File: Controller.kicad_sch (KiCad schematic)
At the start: 28 parts, among them IC3 STM32H563VGT6, U4 BMI088

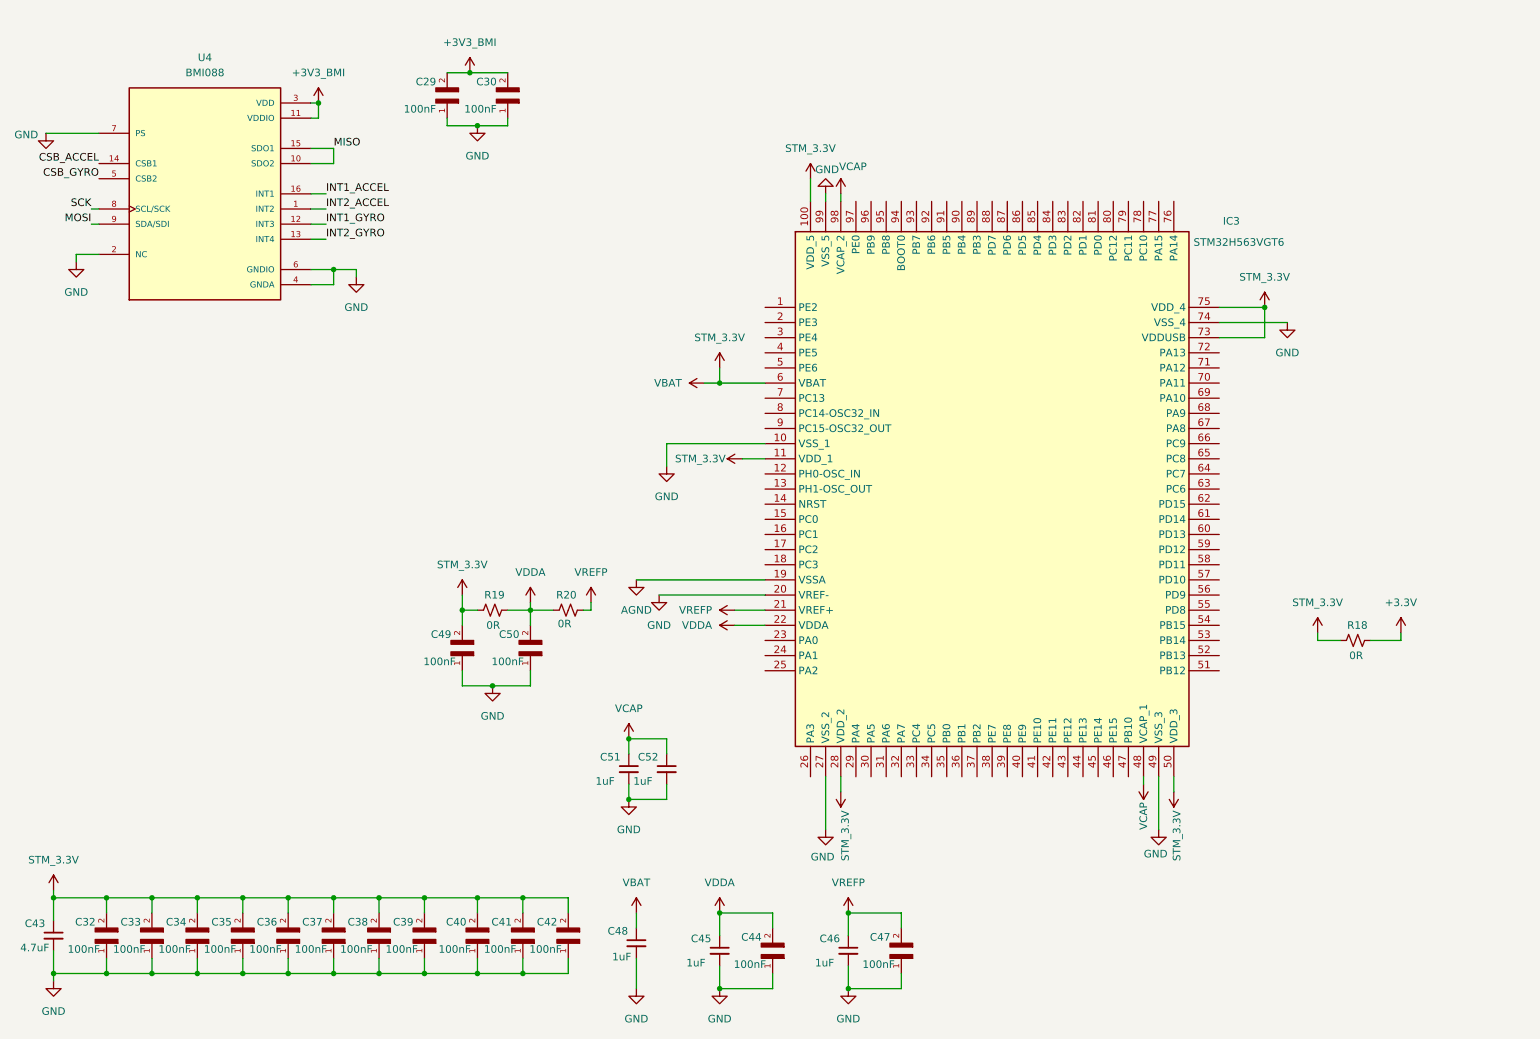
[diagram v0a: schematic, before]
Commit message: new update
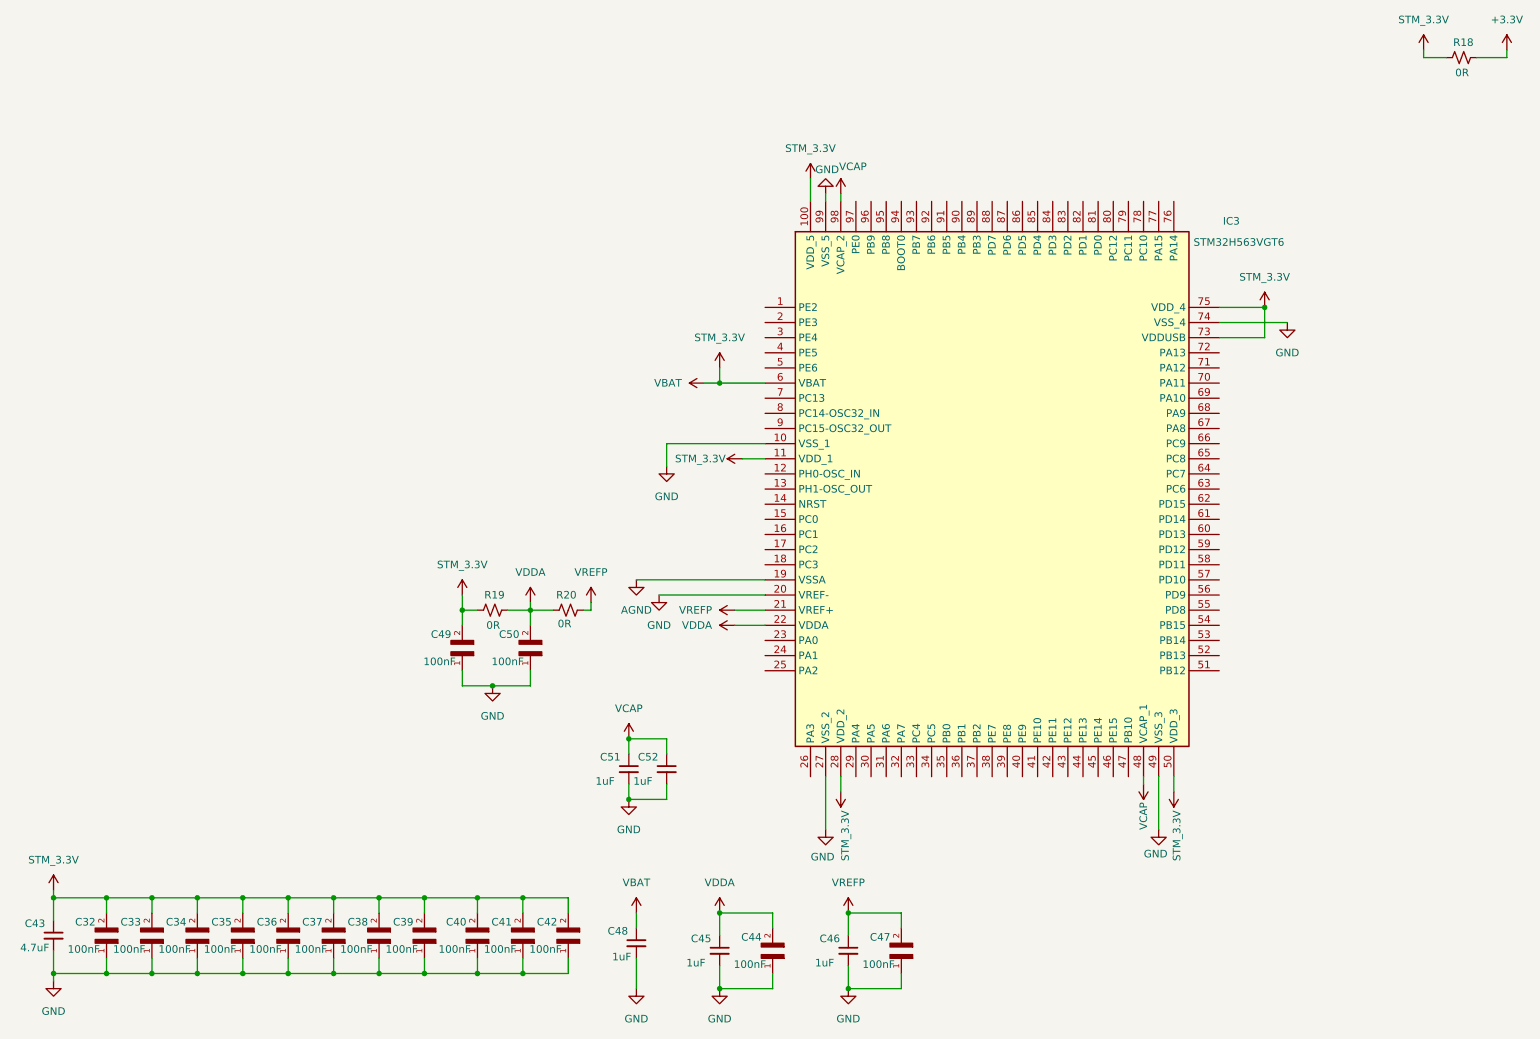
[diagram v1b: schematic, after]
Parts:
- removed C29, C30: 100nF, C0402C104K4RAC:CAPC1005X55N, symbol C0402C104K4RAC:C0402C104K4RAC
- removed U4: BMI088, Module:PQFN50P450X300X100-16N, symbol BMI088:BMI088
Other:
- moved on the sheet: R18

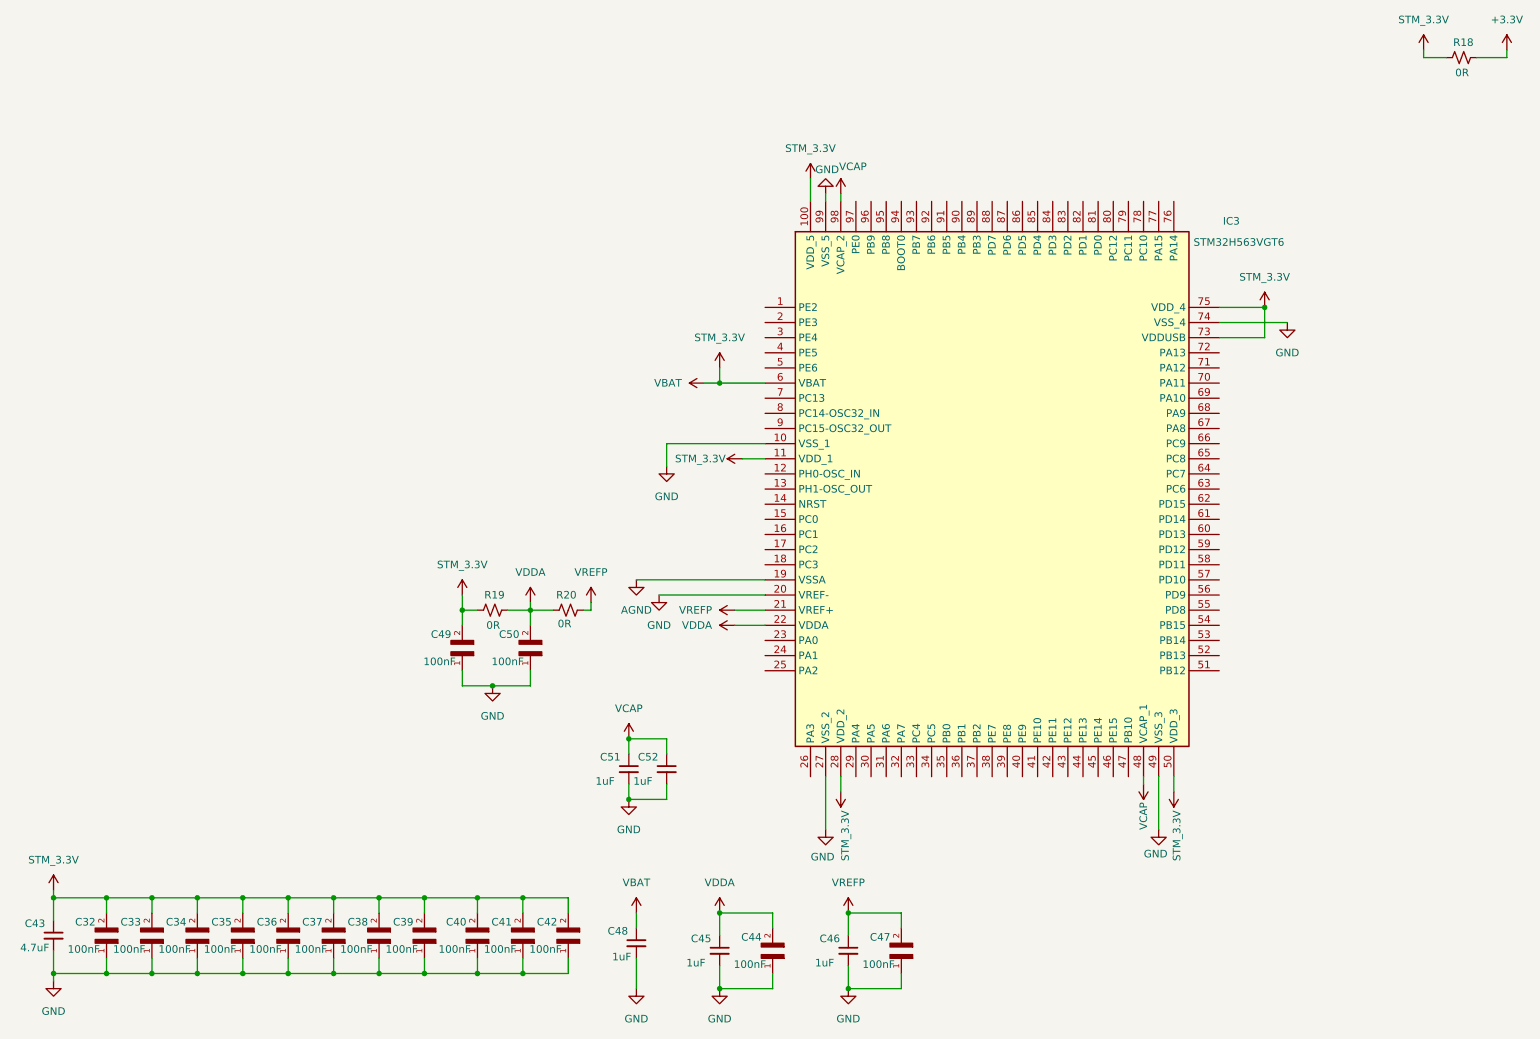
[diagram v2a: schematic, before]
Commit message: new
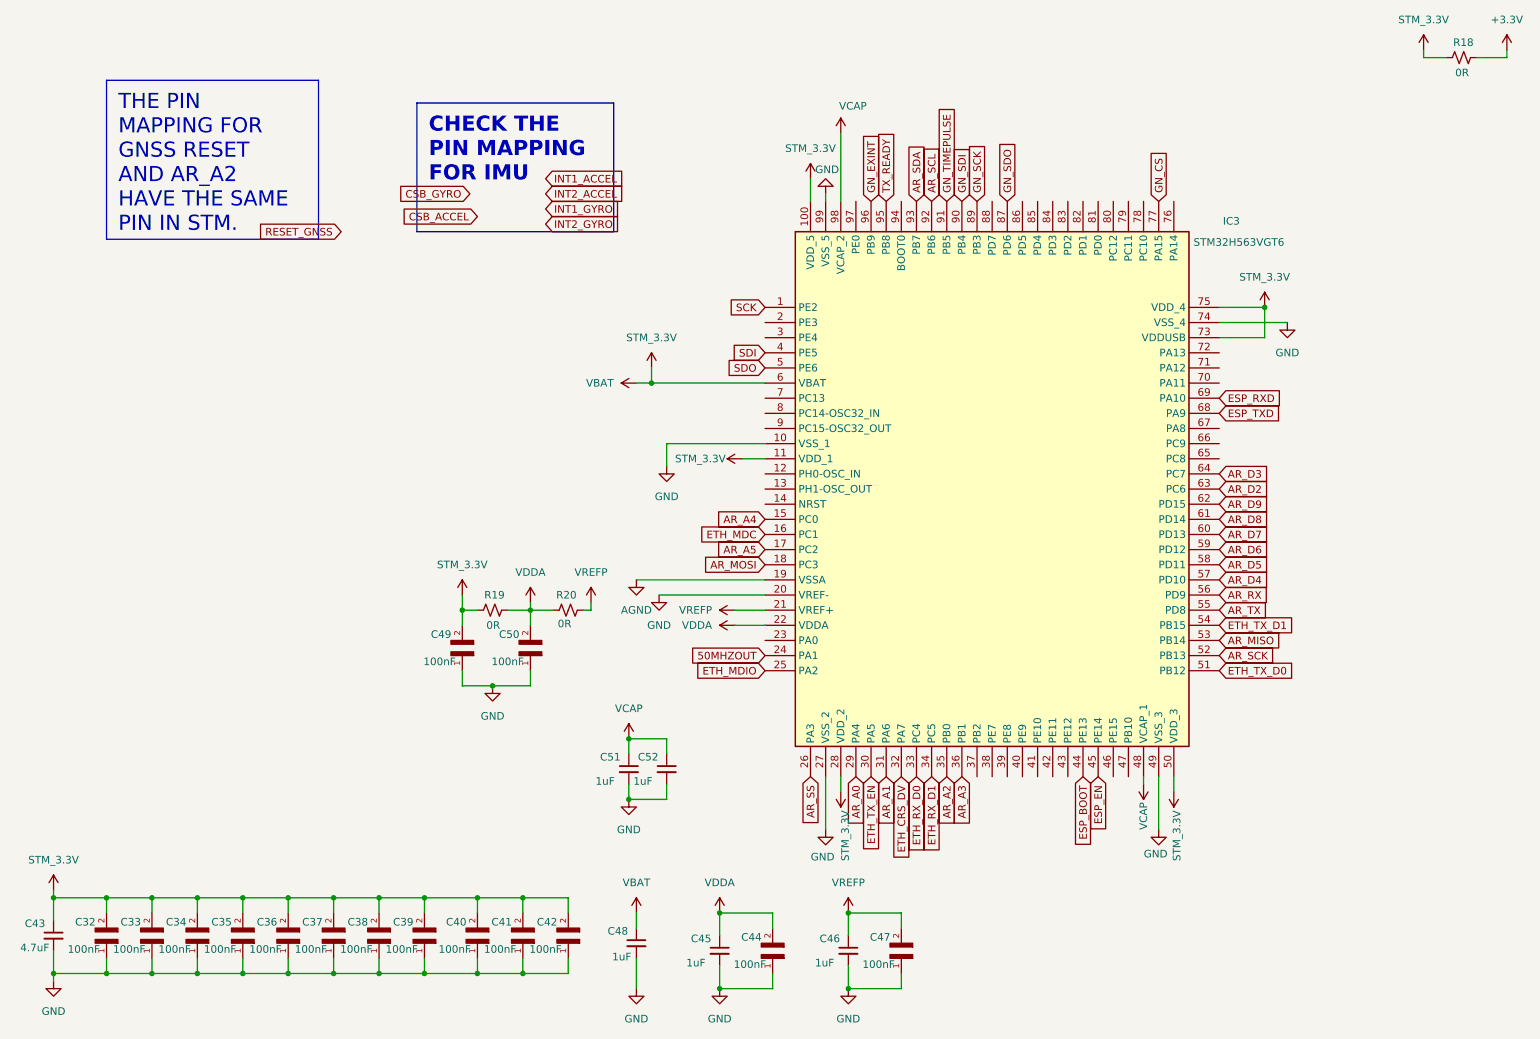
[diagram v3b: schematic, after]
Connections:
- net SCK: now reaches IC3.1 (PE2)
- net AR_A4: now reaches IC3.15 (PC0)
- net ETH_MDC: now reaches IC3.16 (PC1)
- net AR_A5: now reaches IC3.17 (PC2)
- net AR_MOSI: now reaches IC3.18 (PC3)
- net 50MHZOUT: now reaches IC3.24 (PA1)
- net ETH_MDIO: now reaches IC3.25 (PA2)
- net AR_SS: now reaches IC3.26 (PA3)
- net AR_A0: now reaches IC3.29 (PA4)
- net ETH_TX_EN: now reaches IC3.30 (PA5)
- net AR_A1: now reaches IC3.31 (PA6)
- net ETH_CRS_DV: now reaches IC3.32 (PA7)
- net ETH_RX_D0: now reaches IC3.33 (PC4)
- net ETH_RX_D1: now reaches IC3.34 (PC5)
- net AR_A2: now reaches IC3.35 (PB0)
- net AR_A3: now reaches IC3.36 (PB1)
- net SDI: now reaches IC3.4 (PE5)
- net ESP_BOOT: now reaches IC3.44 (PE13)
- net ESP_EN: now reaches IC3.45 (PE14)
- net SDO: now reaches IC3.5 (PE6)
- net ETH_TX_D0: now reaches IC3.51 (PB12)
- net AR_SCK: now reaches IC3.52 (PB13)
- net AR_MISO: now reaches IC3.53 (PB14)
- net ETH_TX_D1: now reaches IC3.54 (PB15)
- net AR_TX: now reaches IC3.55 (PD8)
- net AR_RX: now reaches IC3.56 (PD9)
- net AR_D4: now reaches IC3.57 (PD10)
- net AR_D5: now reaches IC3.58 (PD11)
- net AR_D6: now reaches IC3.59 (PD12)
- net AR_D7: now reaches IC3.60 (PD13)
- net AR_D8: now reaches IC3.61 (PD14)
- net AR_D9: now reaches IC3.62 (PD15)
- net AR_D2: now reaches IC3.63 (PC6)
- net AR_D3: now reaches IC3.64 (PC7)
- net ESP_TXD: now reaches IC3.68 (PA9)
- net ESP_RXD: now reaches IC3.69 (PA10)
- net GN_CS: now reaches IC3.77 (PA15)
- net GN_SDO: now reaches IC3.87 (PD6)
- net GN_SCK: now reaches IC3.89 (PB3)
- net GN_SDI: now reaches IC3.90 (PB4)
- net GN_TIMEPULSE: now reaches IC3.91 (PB5)
- net AR_SCL: now reaches IC3.92 (PB6)
- net AR_SDA: now reaches IC3.93 (PB7)
- net TX_READY: now reaches IC3.95 (PB8)
- net GN_EXINT: now reaches IC3.96 (PB9)
